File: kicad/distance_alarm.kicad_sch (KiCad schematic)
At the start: 10 parts, among them Q1 BC237, U1 RC1602A, U2 PCF8574T

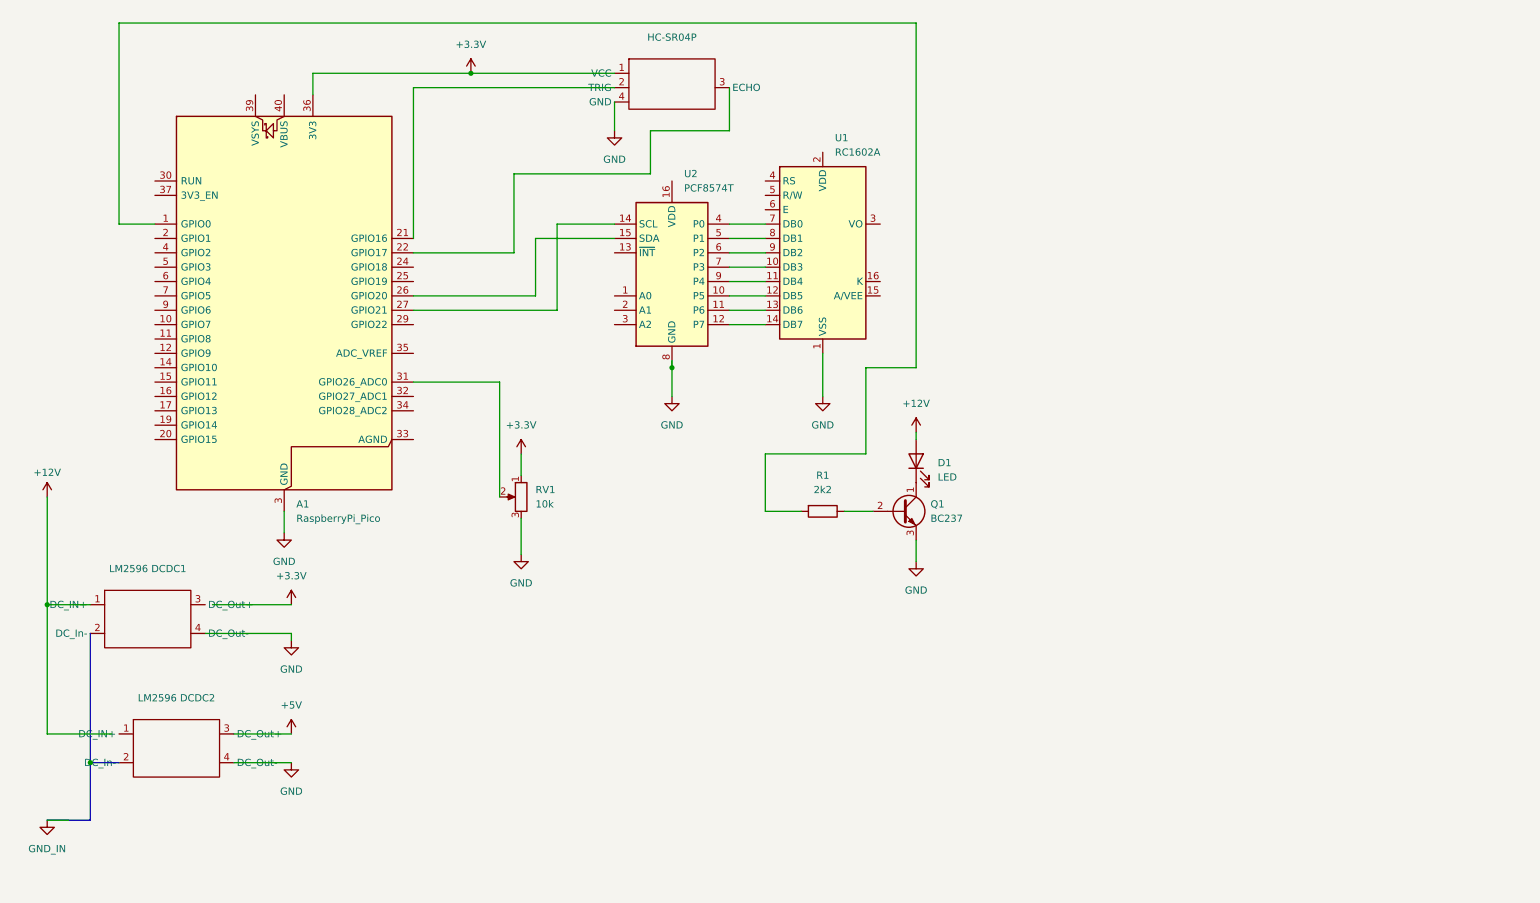
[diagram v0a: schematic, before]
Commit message: Working application
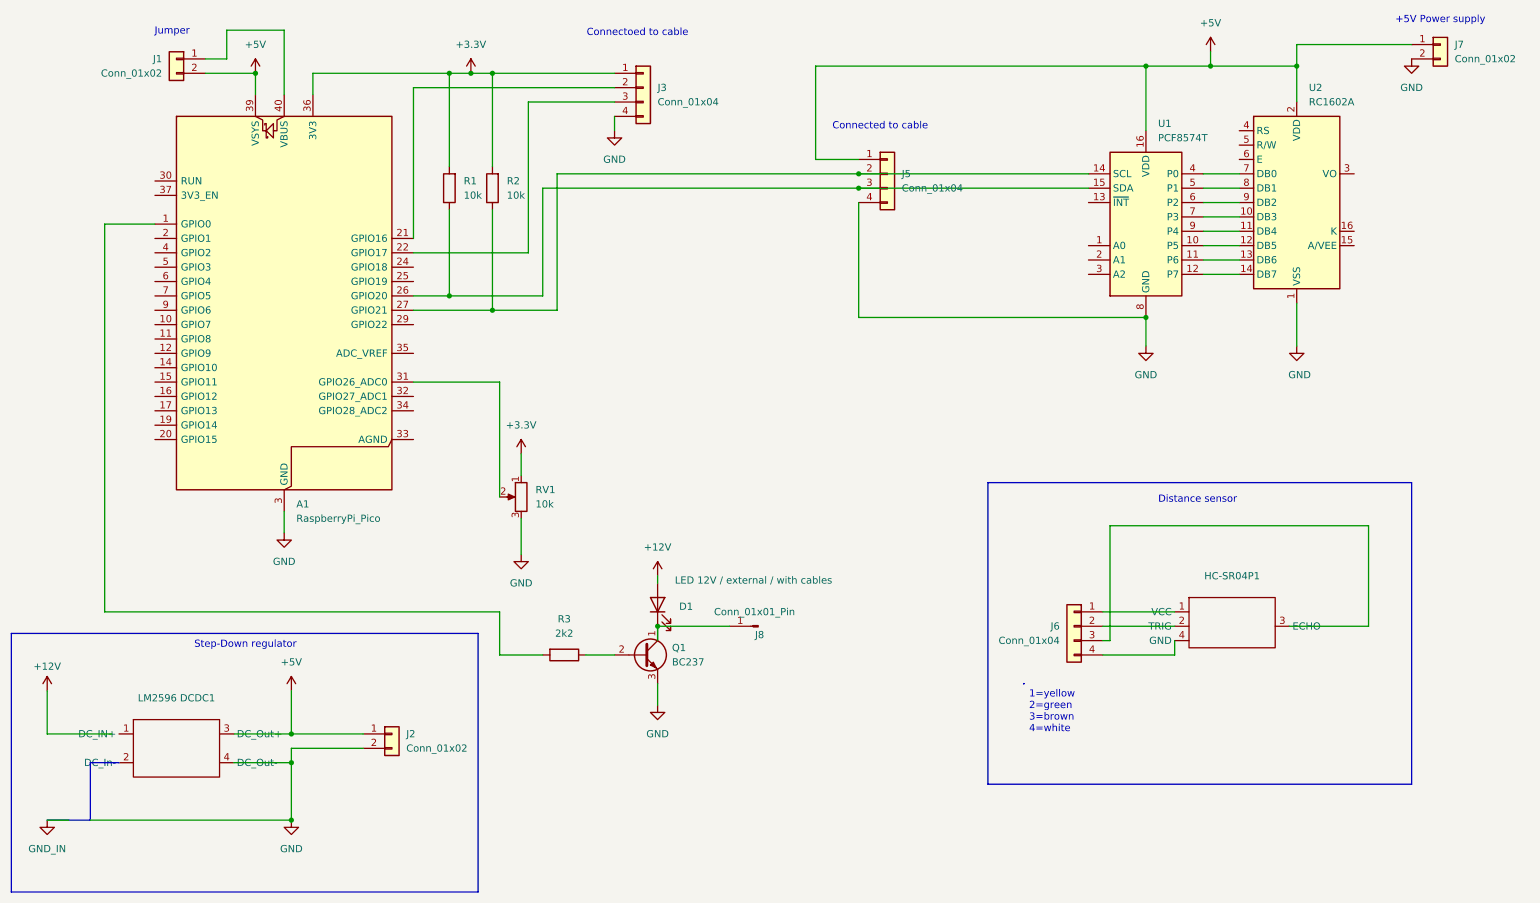
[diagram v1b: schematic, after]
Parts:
- removed LM2596 DCDC1: ~, symbol Converter_DCDC:LM2596_StepDown
- added J1: Conn_01x02, Connector_PinHeader_2.54mm:PinHeader_1x02_P2.54mm_Vertical, symbol Connector_Generic:Conn_01x02
- added J2, J7: Conn_01x02, Connector_PinHeader_2.54mm:PinHeader_1x02_P2.54mm_Horizontal, symbol Connector_Generic:Conn_01x02
- added J3, J5, J6: Conn_01x04, Connector_PinHeader_2.54mm:PinHeader_1x04_P2.54mm_Horizontal, symbol Connector_Generic:Conn_01x04
- added J8: Conn_01x01_Pin, Connector_PinHeader_2.54mm:PinHeader_1x01_P2.54mm_Horizontal, symbol Connector:Conn_01x01_Pin
- added R1, R2: 10k, Resistor_THT:R_Axial_DIN0309_L9.0mm_D3.2mm_P12.70mm_Horizontal, symbol Device:R
- D1: value LED -> LED 12V / external / with cables; footprint (none) -> Connector_PinHeader_2.54mm:PinHeader_1x02_P2.54mm_Horizontal
- LM2596 DCDC1: renamed from LM2596 DCDC2
- R3: renamed from R1; footprint (none) -> Resistor_THT:R_Axial_DIN0309_L9.0mm_D3.2mm_P12.70mm_Horizontal
- RV1: footprint (none) -> Potentiometer_THT:Potentiometer_Piher_PT-10-H05_Horizontal
- renumbered HC-SR04P to HC-SR04P1, U2 to U1, U1 to U2
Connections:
- net +3.3V: now also J3.1 (Pin_1), R1.2, R2.2
- net +5V: now also A1.39 (VSYS), U1.16 (VDD), U2.2 (VDD), J1.2 (Pin_2), J2.1 (Pin_1), J5.1 (Pin_1), J7.1 (Pin_1)
- net GND: now also J2.2 (Pin_2), J3.4 (Pin_4), J5.4 (Pin_4), J7.2 (Pin_2)
- net at D1.1 (K), Q1.1 (C): now also J8.1 (Pin_1)
- net at A1.21 (GPIO16): now also J3.2 (Pin_2)
- net at A1.22 (GPIO17): now also J3.3 (Pin_3)
- net at A1.26 (GPIO20), U1.15 (SDA): now also J5.3 (Pin_3), R1.1
- net at A1.27 (GPIO21), U1.14 (SCL): now also J5.2 (Pin_2), R2.1
- net at A1.40 (VBUS): now also J1.1 (Pin_1)
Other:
- note added: "+5V Power supply"
- note added: "Connected to cable"
- note added: "Connectoed to cable"
- note added: "Distance sensor"
- note added: "Jumper"
- note added: "Step-Down regulator"
- moved on the sheet: D1, HC-SR04P1, Q1, R3, U1, U2
